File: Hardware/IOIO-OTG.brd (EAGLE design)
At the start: 68.6 x 30.5 mm, 54 parts, among them Q1 IRLML2244, Q2 MOSFET-NCHANNEL2N7002PW", U1 PIC24FJ256GB206, U14 SWITCH_SPDT, U2 TPS6214X"", U3 VREG_MIC5216

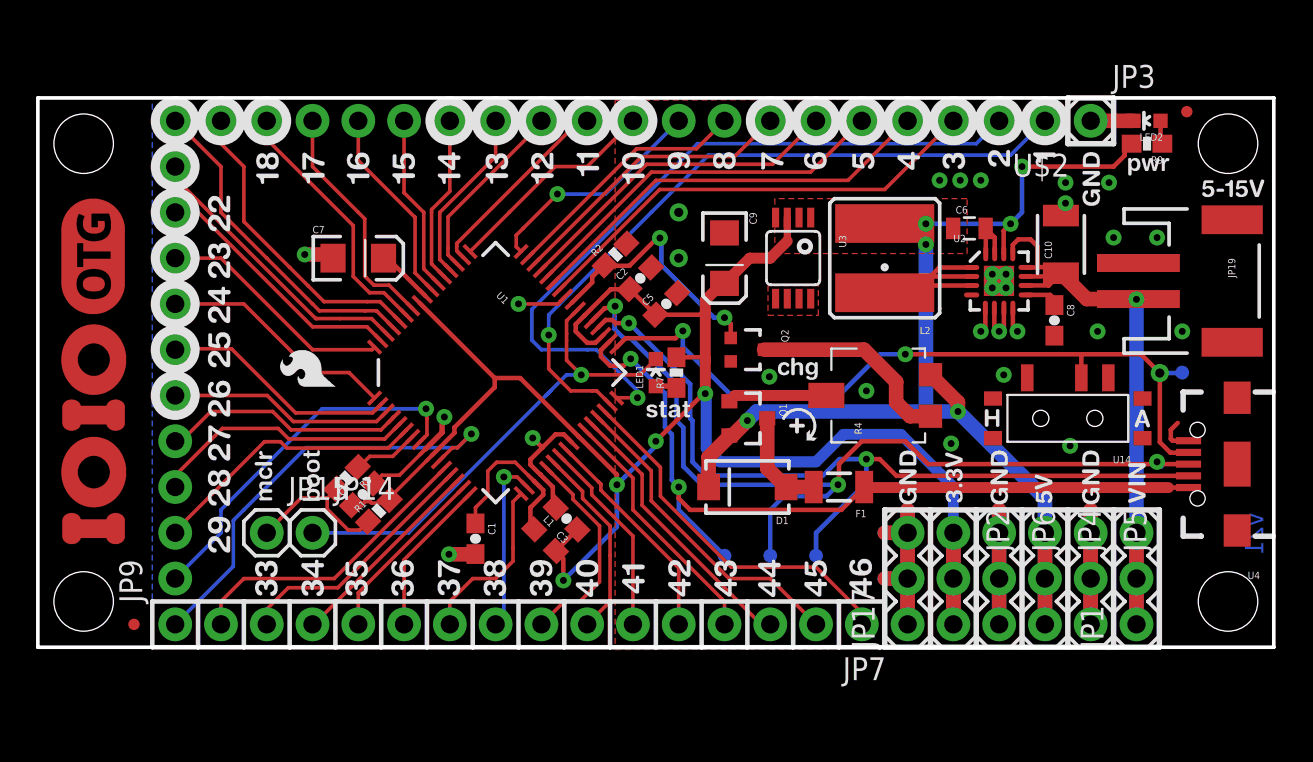
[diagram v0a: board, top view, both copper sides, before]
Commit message: Adding in hardware changes from Pete
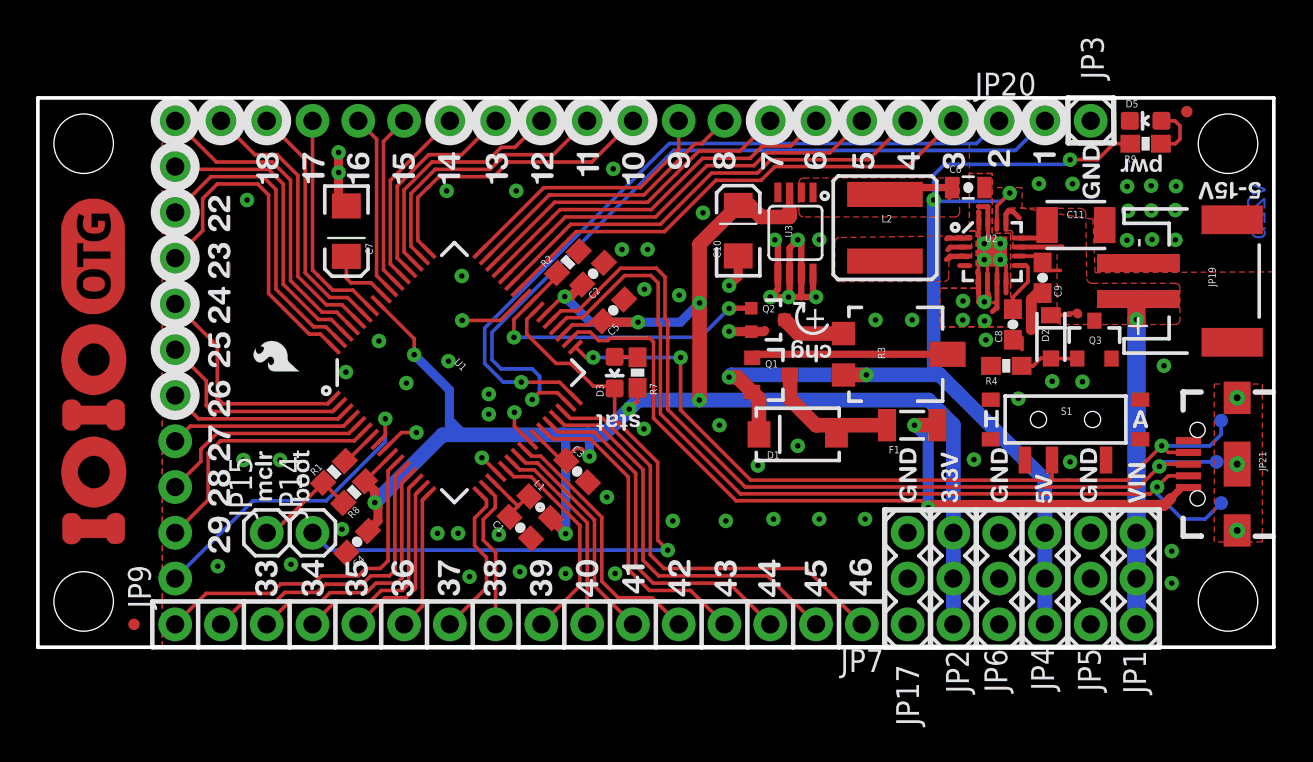
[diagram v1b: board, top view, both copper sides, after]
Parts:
- removed LED1: LY L29K-J1K2-26-Z, SparkFun-LED:LED-0603
- removed LED2: LS L29K-G1J2-1-Z, SparkFun:LED-0603
- removed TP4: TEST-POINT3, SparkFun-Passives:PAD.03X.03
- removed U$1: CREATIVE_COMMONS, SparkFun-Aesthetics:CREATIVE_COMMONS
- removed U14: SWITCH_SPDT, SparkFun-Electromechanical:KPS-1290
- removed U4: (no value), Testing:USB-AB-MICRO-SMD_V03
- added C11: 10uF, SparkFun-Capacitors:1210
- added D2: DZ2J160M0L, SparkFun-DiscreteSemi:PANASONIC_SMINI2-F5-B
- added D3: Yellow, SparkFun-LED:LED-0603
- added D5: Red, SparkFun-LED:LED-0603
- added FRAME2: FRAME-LEDGER, SparkFun-Aesthetics:CREATIVE_COMMONS
- added JP21: AB MICRO USB, SparkFun-Connectors:USB-AB-MICRO-SMD_V03
- added LOGO1: OSHW-LOGOS, SparkFun-Aesthetics:OSHW-LOGO-S
- added LOGO2: SFE_LOGO_NAME_FLAME.1_INCH, SparkFun-Aesthetics:SFE_LOGO_NAME_FLAME_.1
- added LOGO3: SFE_LOGO_FLAME.1_INCH, SparkFun-Aesthetics:SFE_LOGO_FLAME_.1
- added Q3: MOSFET-NCHANNELAO3404A, SparkFun-DiscreteSemi:SOT23-3
- added R3: TS53YL502MR10, SparkFun-Electromechanical:TRIMPOT_5MM
- added S1: SWITCH_SPDT, SparkFun-Electromechanical:KPS-1290
- C10: value 10uf -> 10uF; device SparkFun-Passives:1210 -> SparkFun-Capacitors:EIA3216
- C6: value 10uf -> 10uF; device SparkFun-Passives:0805 -> SparkFun-Capacitors:0805-CAP
- C7: device SparkFun:EIA3216 -> SparkFun-Capacitors:EIA3216
- C9: value 10uf -> 0.1uF; device SparkFun-Capacitors:EIA3216 -> SparkFun-Capacitors:0603-CAP
- D1: value DIODE-SCHOTTKY_ -> B340A
- F1: value PTCSMD -> 0.75A
- JP1: value VIN -> (none)
- JP14, JP15, JP3: value M01PTH -> (none)
- JP19: value JST Connector -> JST; device SparkFun:JST-2-SMD -> SparkFun-Connectors:JST-2-SMD
- JP20: value M191X19_NO_SILK -> (none)
- JP4: value 5V -> (none)
- JP7: value M161X16_NO_SILK -> (none)
- JP9: value M111X11_NO_SILK -> (none)
- Q2: value MOSFET-NCHANNEL2N7002PW" -> 2N7002PW; device SparkFun-DiscreteSemi:SOT323_NOAT -> SparkFun-DiscreteSemi:SOT323
- R1: value 10k -> 10K
- R4: value TRIMPOTSMD_STANDARD -> 3.3k; device Testing:TRIMPOT_5MM -> SparkFun-Resistors:0603-RES
- R9: value 1.6k -> 1.6K
- U2: value TPS6214X"" -> TPS62133RGTT
- U3: value VREG_MIC5216 -> MIC5216
- moved TP1 28.6 mm to (65.7, 12.6)
- moved TP3 25.2 mm to (65.7, 8.00)
- moved TP2 22.8 mm to (65.4, 10.3)
- moved C10 17.9 mm to (38.9, 23.1)
- moved C9 17.7 mm to (55.8, 20.5)
- moved R4 6.94 mm to (53.7, 15.6), turned to 180 degrees
- moved F1 5.32 mm to (48.5, 12.3)
- moved D1 4.04 mm to (42.2, 11.8)
- moved C5 2.97 mm to (31.9, 18.7)
- moved Q1 2.73 mm to (40.6, 15.1)
- moved C3 2.68 mm to (29.9, 9.75), turned to 315 degrees
- moved R2 2.68 mm to (29.4, 21.4)
- moved C4 2.65 mm to (17.7, 5.85), turned to 225 degrees
- moved C2 2.63 mm to (30.8, 20.7)
- moved C1 2.56 mm to (26.8, 6.63), turned to 315 degrees
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- renumbered U$2 to JP20
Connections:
- new net ANCHOR1: JP21.SHIELD1, JP21.SHIELD2, JP21.SHIELD3
- new net N$12: D2.A, Q3.1, R4.1
- net 3.3V: now also C10.A; no longer C9.A
- net 5V: now also R3.A; no longer R4.A
- net BOOT: now also D3.C; no longer LED1.C
- net D+: now also JP21.D+1, TP2.P$1; no longer TP3.P$1, U4.D+1
- net D-: now also JP21.D-1, TP3.P$1; no longer TP2.P$1, U4.D-1
- net GND: now also C10.C, C11.2, C9.2, D5.C, JP21.GND1, Q3.2, R4.2, S1.S; no longer C10.2, C9.C, LED2.C, U14.O, U4.GND1
- net N$1: now also R3.B; no longer R4.B
- net N$2: now also D3.A; no longer LED1.A
- net N$3: now also D5.A; no longer LED2.A
- net N$8: now also R3.C; no longer R4.C
- net USBID: now also JP21.ID1, S1.P, TP1.P$1; no longer TP4.P$1, U14.P, U4.ID1
- net VBUS: now also JP21.VBUS1; no longer TP1.P$1, U4.VBUS1
- net VIN: now also C11.1, C9.1, D2.C, Q3.3; no longer C10.1
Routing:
- net GND: track 74.9 -> 52.1 mm, vias 29 -> 82
- net BOOT: track 27.7 -> 38.1 mm
- net VIN: track 38.7 -> 28.5 mm
- net 3.3V: track 101.7 -> 111.4 mm, vias 4 -> 9
- net N$8: track 11.4 -> 3.58 mm
- net N$6: track 10.5 -> 3.14 mm
- net N$9: track 9.66 -> 3.63 mm
- net PIN31: track 24.8 -> 19.0 mm, vias 1 -> 0
- net N$1: track 5.51 -> 10.9 mm
- net PIN23: track 13.2 -> 18.5 mm
- net PIN10: track 12.0 -> 17.0 mm
- net PIN1: track 39.2 -> 44.0 mm
- net HOST: track 14.1 -> 18.6 mm
- net D-: track 46.3 -> 50.8 mm, vias 2 -> 1
- net PIN44: track 15.6 -> 19.8 mm
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- added copper zone on layer 1, net ANCHOR1
- added copper zone on layer 1, net N$6
- added copper zone on layer 1, net VIN
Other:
- board text added: "+"
- board text added: "Aaron Weiss, Pete Lewis"
- board text added: "Revised by:"
- board text added: "Units are in inches"
- board text added: "Ytai Ben-tsvi"
- board text added: "v22b"
- board text removed: "D+"
- board text removed: "D-"
- board text removed: "ID"
- board text removed: "VBUS"
- board text removed: "v21"
